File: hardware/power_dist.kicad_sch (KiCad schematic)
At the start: 10 parts, among them U1 TPS62175DQC

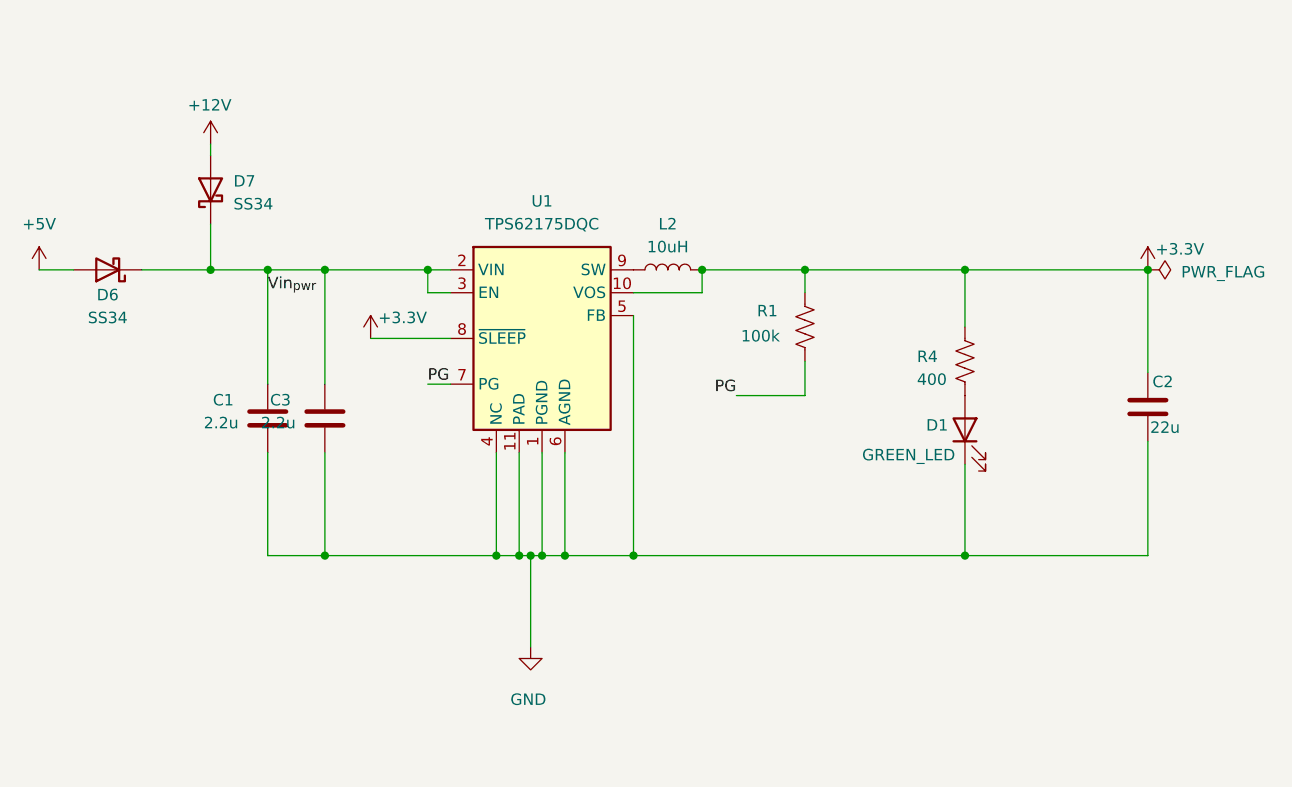
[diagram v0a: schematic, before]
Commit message: resolved comments
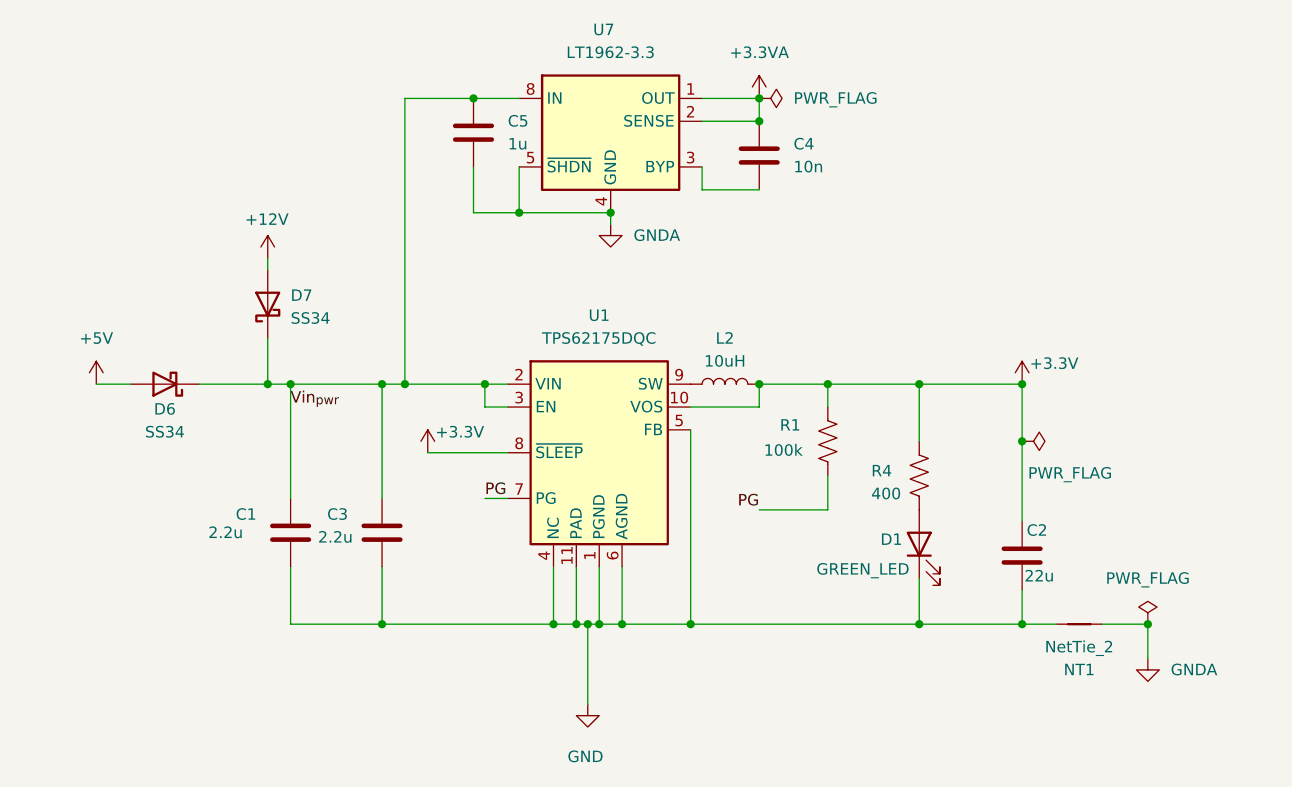
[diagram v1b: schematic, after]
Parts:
- added C4: 10n, Capacitor_SMD:C_0603_1608Metric, symbol Device:C
- added C5: 1u, Capacitor_SMD:C_0603_1608Metric, symbol Device:C
- added NT1: NetTie_2, NetTie:NetTie-2_THT_Pad1.0mm, symbol Device:NetTie_2
- added U7: LT1962-3.3, Package_SO:MSOP-8_3x3mm_P0.65mm, symbol Regulator_Linear:LT1962-3.3
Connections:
- net GND: now also NT1.2
- net Vin_{pwr}: now also C5.1, U7.8 (IN)
- new net: C4.2, U7.3 (BYP)
- new net +3.3VA: C4.1, U7.1 (OUT), U7.2 (SENSE)
- new net GNDA: C5.2, NT1.1, U7.4 (GND), U7.5 (~{SHDN})
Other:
- moved on the sheet: C1, C2, C3, D1, D6, D7, L2, R1, R4, U1
